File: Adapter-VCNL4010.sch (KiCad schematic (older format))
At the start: 8 parts, among them J1 Conn_01x03, J2 Conn_01x03, U1 VCNL4010

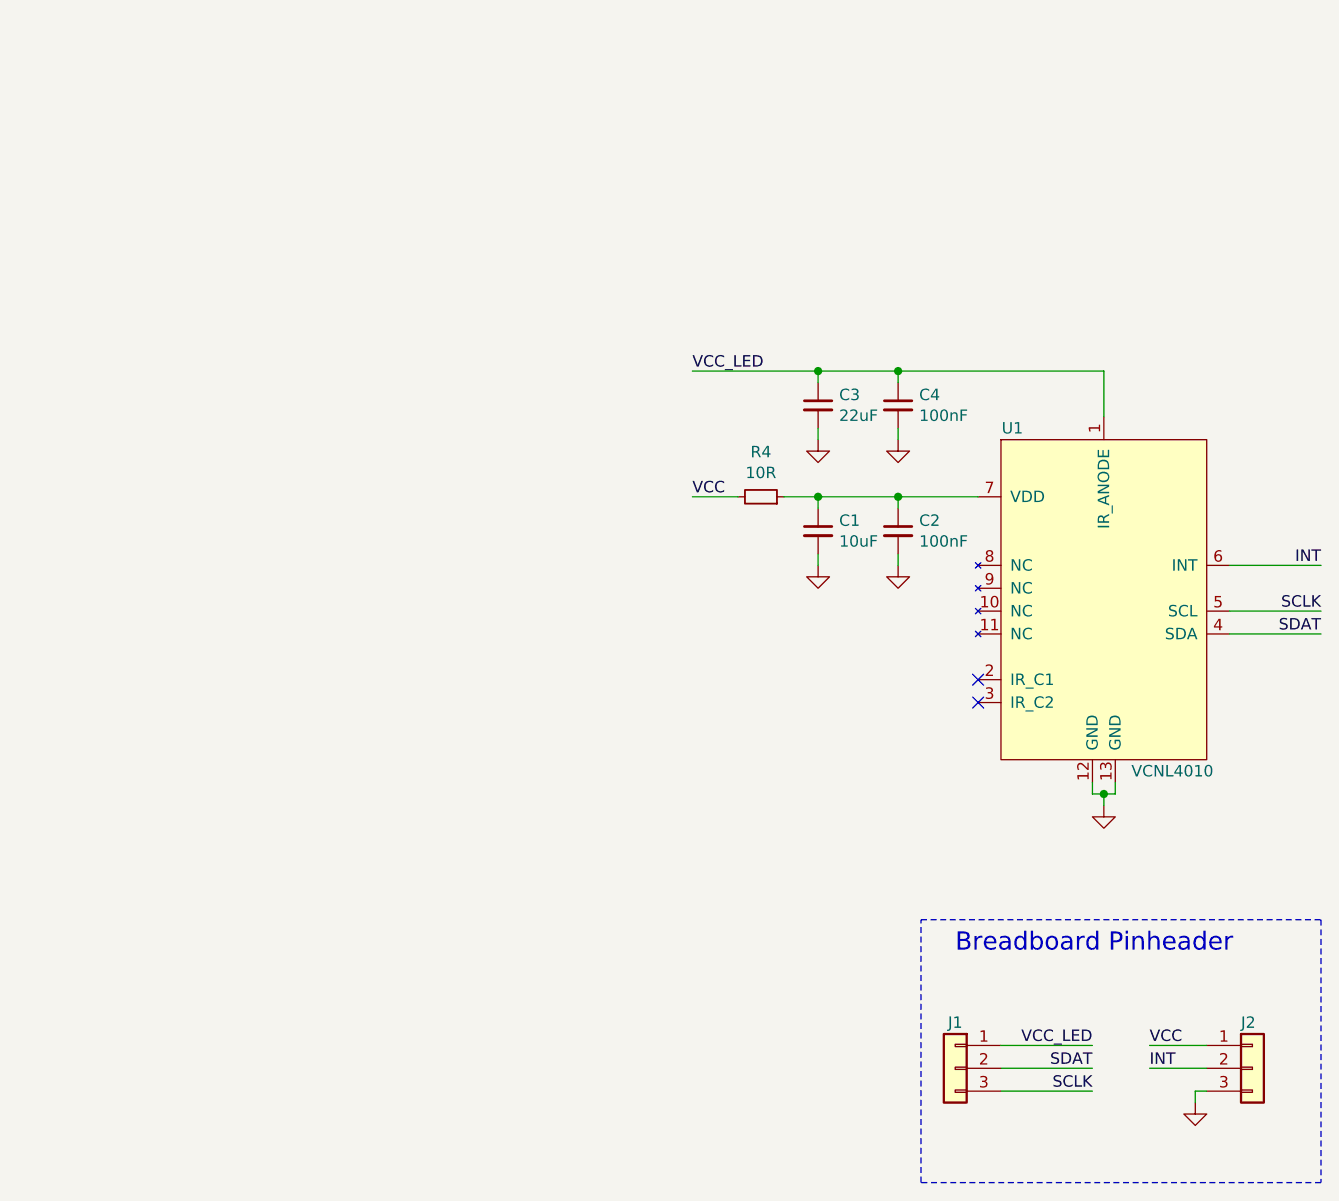
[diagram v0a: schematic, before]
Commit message: added PDF
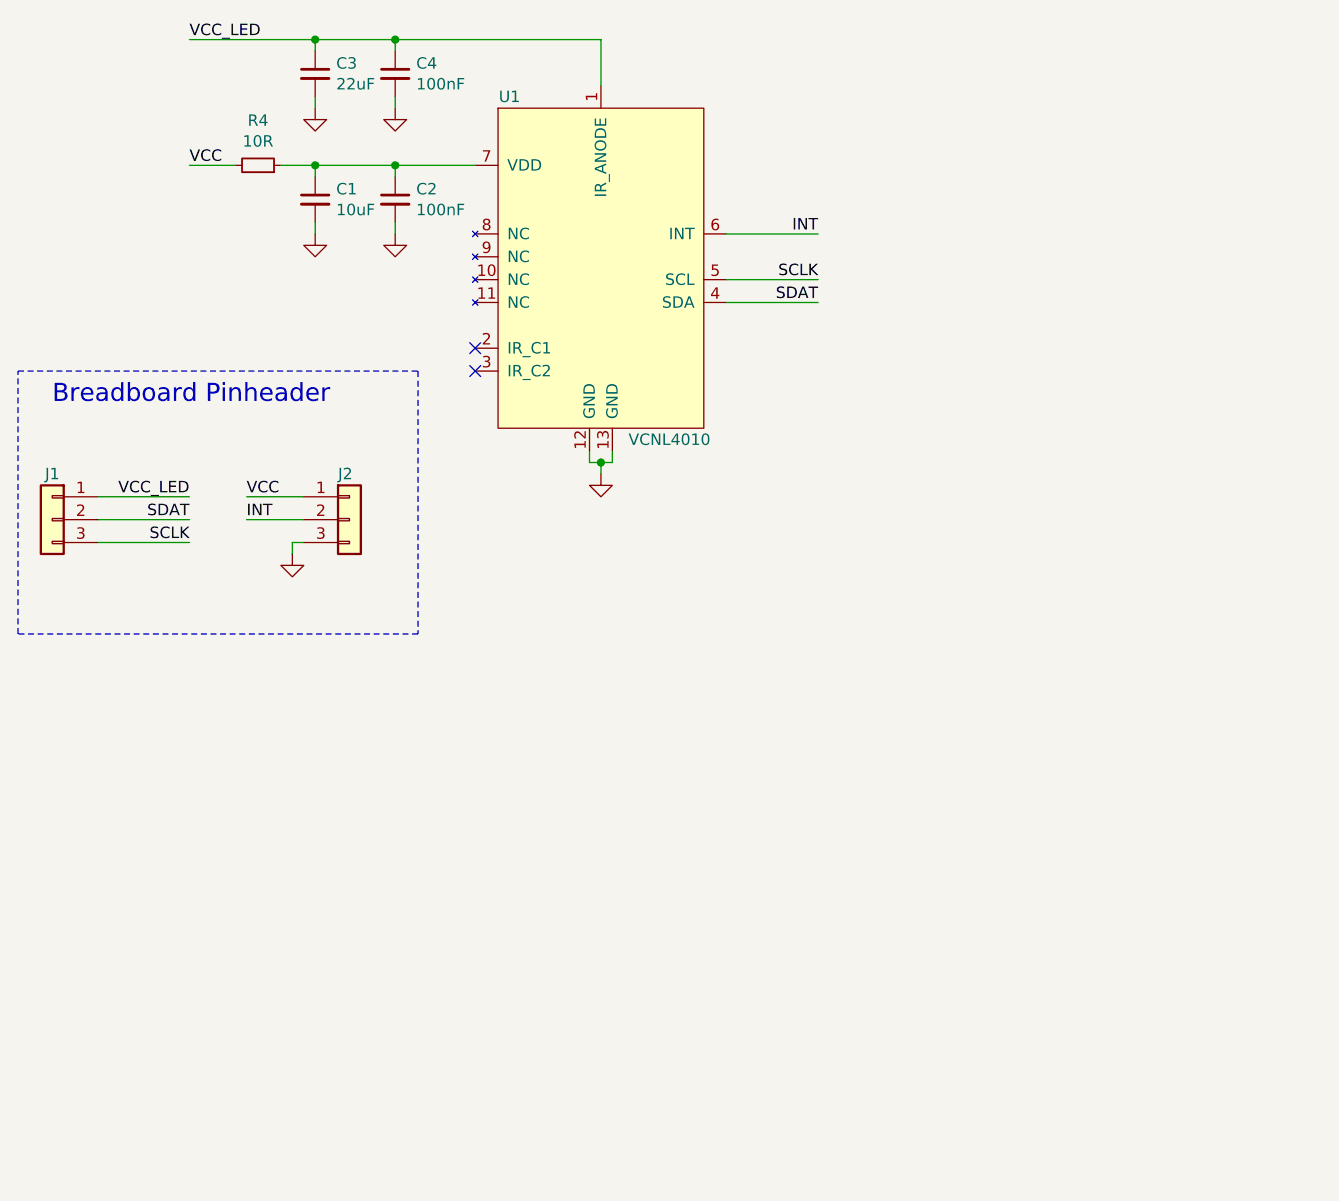
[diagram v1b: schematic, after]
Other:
- moved on the sheet: C1, C2, C3, C4, J1, J2, R4, U1
